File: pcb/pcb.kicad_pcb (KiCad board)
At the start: 2 copper layers, 68.2 x 24.6 mm, 27 parts, among them U1 ATtiny85-20P, U2 FS8205A, U3 TP4056, U4 DW01A, U5 AMS1117-5.0

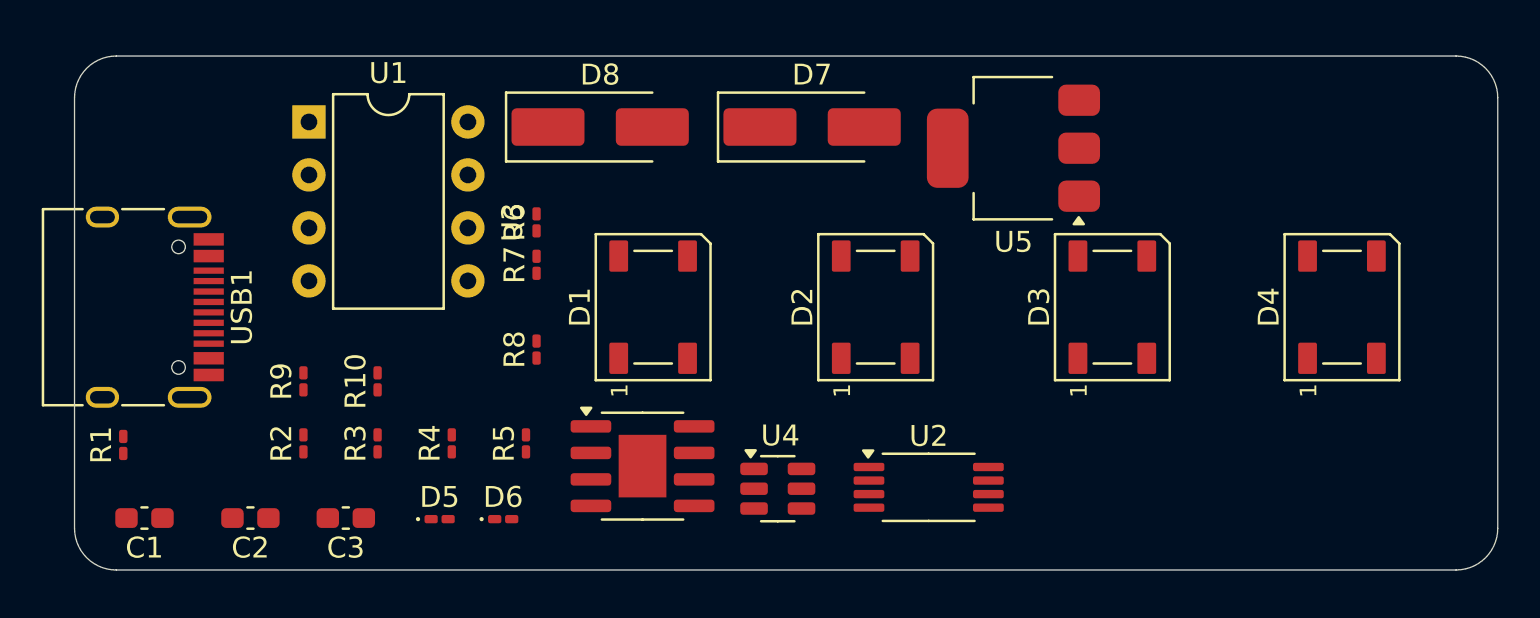
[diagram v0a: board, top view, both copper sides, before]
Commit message: route
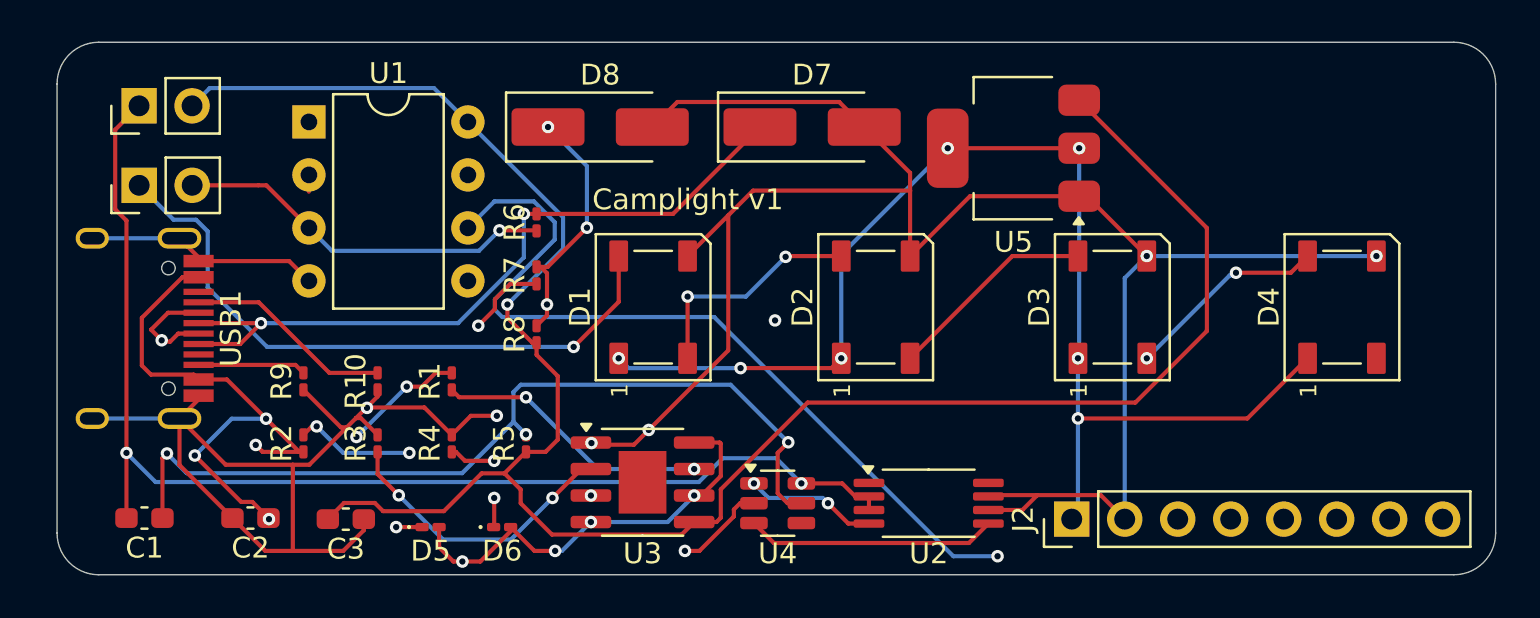
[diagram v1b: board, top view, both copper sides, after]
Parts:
- added J1: Conn_01x02_Pin, Connector_PinHeader_2.54mm:PinHeader_1x02_P2.54mm_Vertical, F.Cu at (59.2, 53.8)
- added J2: Conn_01x08_Pin, Connector_PinHeader_2.54mm:PinHeader_1x08_P2.54mm_Vertical, F.Cu at (103.9, 73.7)
- added J3: Conn_01x02_Pin, Connector_PinHeader_2.54mm:PinHeader_1x02_P2.54mm_Vertical, F.Cu at (59.2, 57.7)
- USB1: footprint Connector_USB:USB_C_Receptacle_HRO_TYPE-C-31-M-12 -> USB-C:HRO-TYPE-C-31-M-12
- moved R1 16.0 mm to (74.2, 67.1)
- moved USB1 4.26 mm to (54.3, 64.5)
- moved U3 0.77 mm to (83.3, 71.9)
- moved U2 0.76 mm to (97.0, 72.9)
- moved R8 0.74 mm to (78.2, 64.8)
- moved U4 0.70 mm to (89.8, 72.9)
- moved D5 0.58 mm to (73.2, 74.0)
- moved R7 0.51 mm to (78.2, 62.0)
- moved D6 0.38 mm to (76.6, 74.0)
- moved C3 0.05 mm to (69.1, 73.7)
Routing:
- net OUT-: track 0.00 -> 168.9 mm, vias 0 -> 7
- net OUT+: track 0.00 -> 100.2 mm, vias 0 -> 1
- net Net-(D5-A): track 0.00 -> 64.7 mm, vias 0 -> 8
- net +5V: track 0.00 -> 59.7 mm, vias 0 -> 7
- net Net-(J2-Pin_5): track 0.00 -> 59.0 mm, vias 0 -> 1
- net Net-(J2-Pin_4): track 0.00 -> 59.0 mm, vias 0 -> 2
- net Net-(J2-Pin_7): track 0.00 -> 59.0 mm, vias 0 -> 1
- net Net-(J1-Pin_1): track 0.00 -> 58.5 mm, vias 0 -> 2
- net Net-(J2-Pin_3): track 0.00 -> 51.7 mm
- net Net-(J2-Pin_8): track 0.00 -> 51.5 mm
- net Net-(J2-Pin_6): track 0.00 -> 48.5 mm
- net Net-(U4-VCC): track 0.00 -> 41.9 mm, vias 0 -> 3
- net D-: track 0.00 -> 37.2 mm, vias 0 -> 4
- net D+: track 0.00 -> 35.4 mm, vias 0 -> 2
- net Net-(D1-DIN): track 0.00 -> 30.9 mm, vias 0 -> 1
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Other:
- board size 68.2 x 24.6 mm -> 69 x 25.5 mm
- copper layers 2 -> 4
- board text added: "Camplight v1"
